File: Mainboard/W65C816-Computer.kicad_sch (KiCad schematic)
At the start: 93 parts, among them J1 ADDR_DATA_DBG, J2 CTRL_BANK_DBG, J3 CPU_MISC_DBG, J4 PJ-102A, J5 DAUGHTER_PWR_AUX, J6 DAUGHTER_BUS_A, J7 DAUGHTER_BUS_B, Q1 P-MOSFET_REV_PROT_TO220, SW1 RESET, SW2 NMI, SW3 MAIN_PWR_SW_EXT, U1 W65C816S6PG-14, U10 SN74HC04N, U2 SN74HC573N, U20 AS6C4008-55PCN, U21 AS6C4008-55PCN, U22 AS6C4008-55PCN, U23 AS6C4008-55PCN, U24 AS6C4008-55PCN, U25 AS6C4008-55PCN, U26 AS6C4008-55PCN, U27 AS6C4008-55PCN, U3 SN74HC245N, U30 SST39VF040-70-4I-NHE, U4 MCP130-315D, U5 SN74HC14N, U6 SN74HC138N, U7 SN74HC138N, U9 SN74HC00N, X1 ECS-P143X-8.000-BN

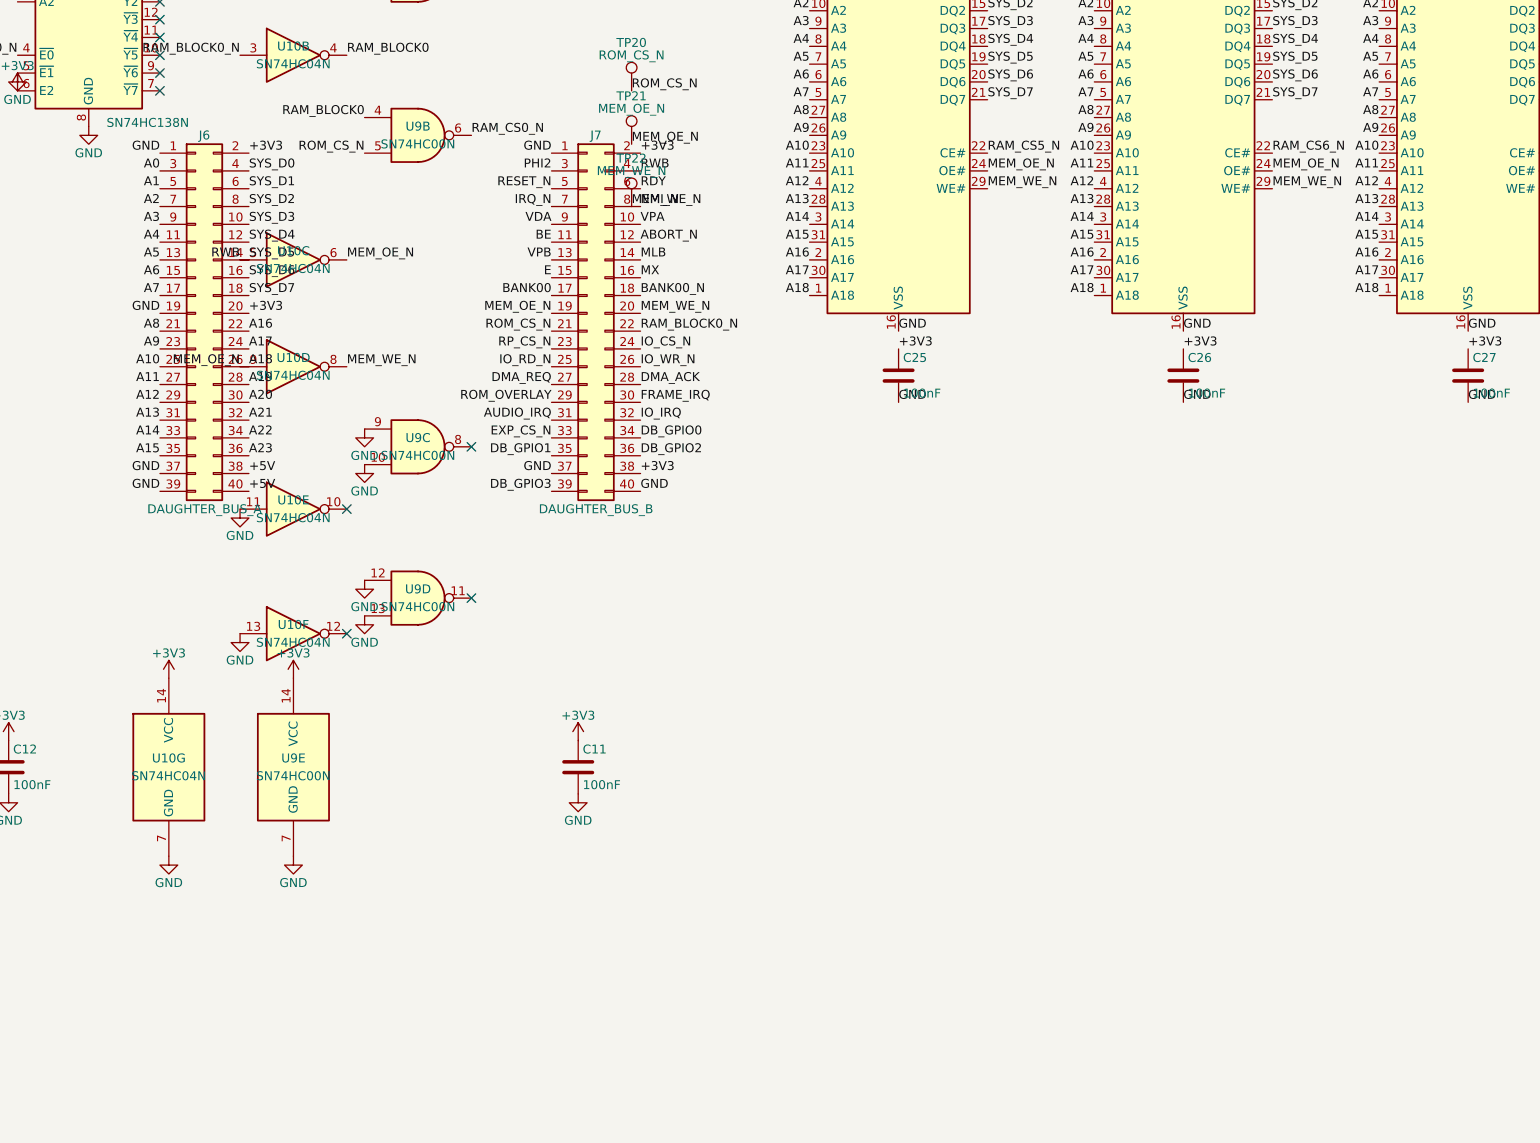
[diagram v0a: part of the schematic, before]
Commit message: Add lock file for W65C816-Computer project with hostname and username
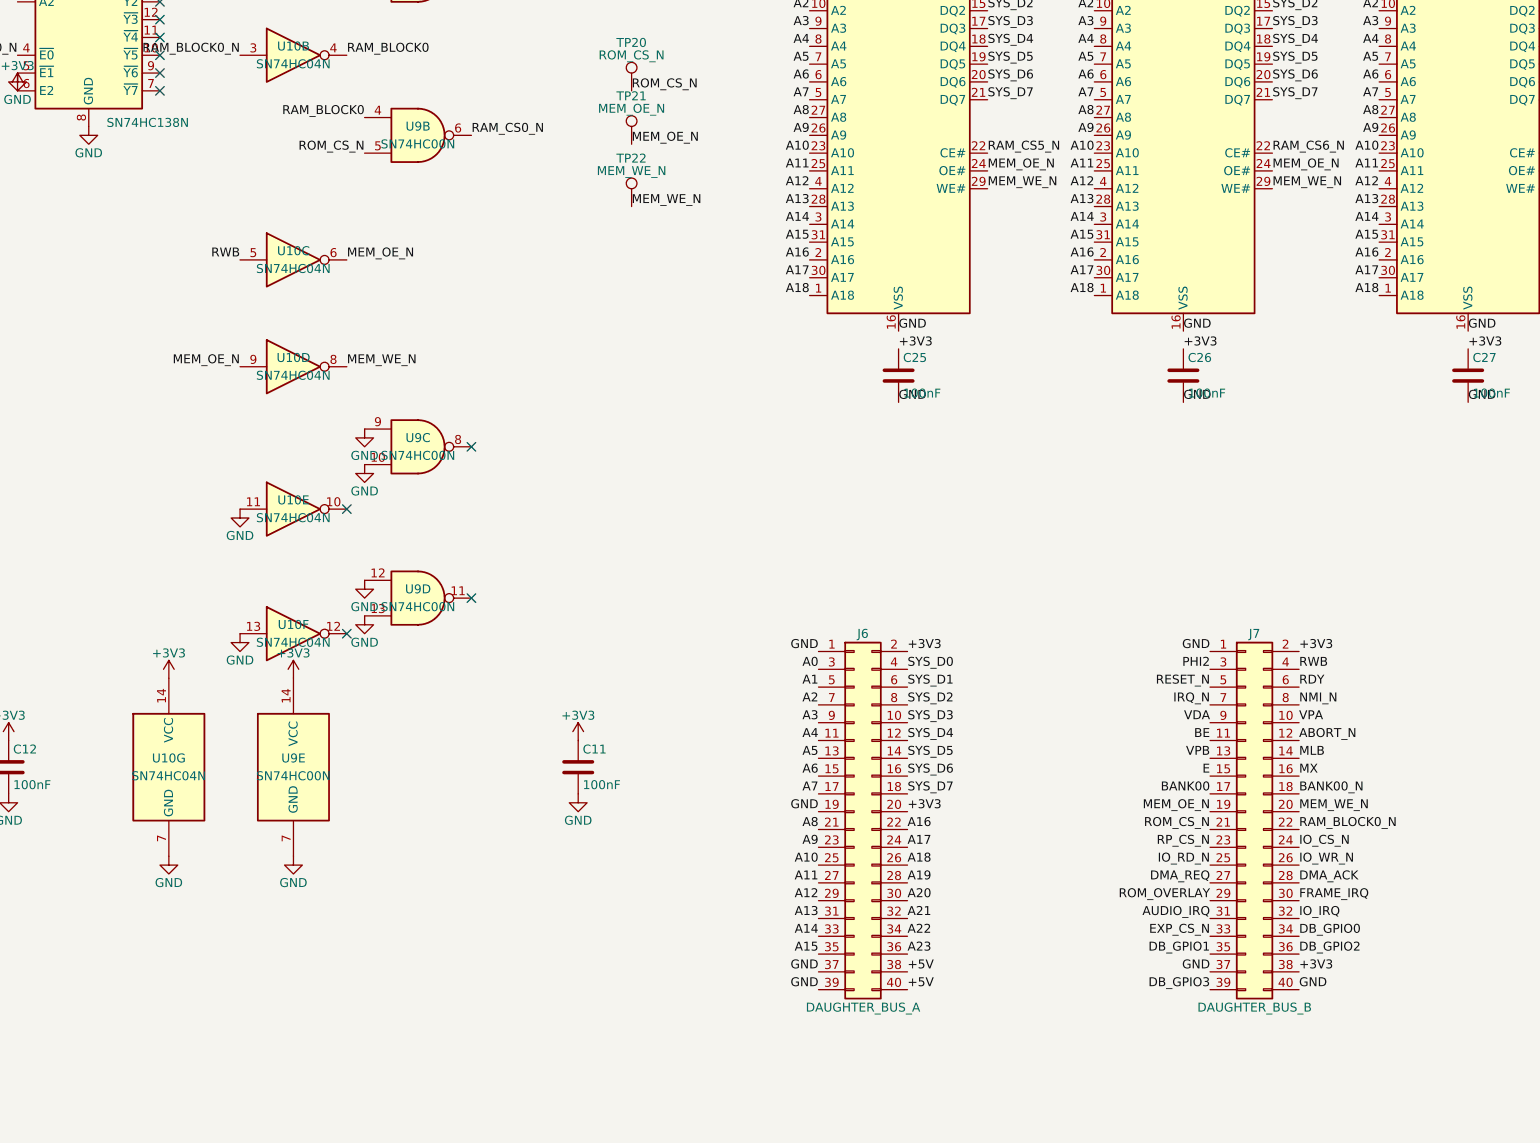
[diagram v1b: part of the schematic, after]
